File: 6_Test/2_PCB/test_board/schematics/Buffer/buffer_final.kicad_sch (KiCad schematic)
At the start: 12 parts, among them J11 Buffer_PWR_Jumper, U7 SN74ALVCH162827DLR

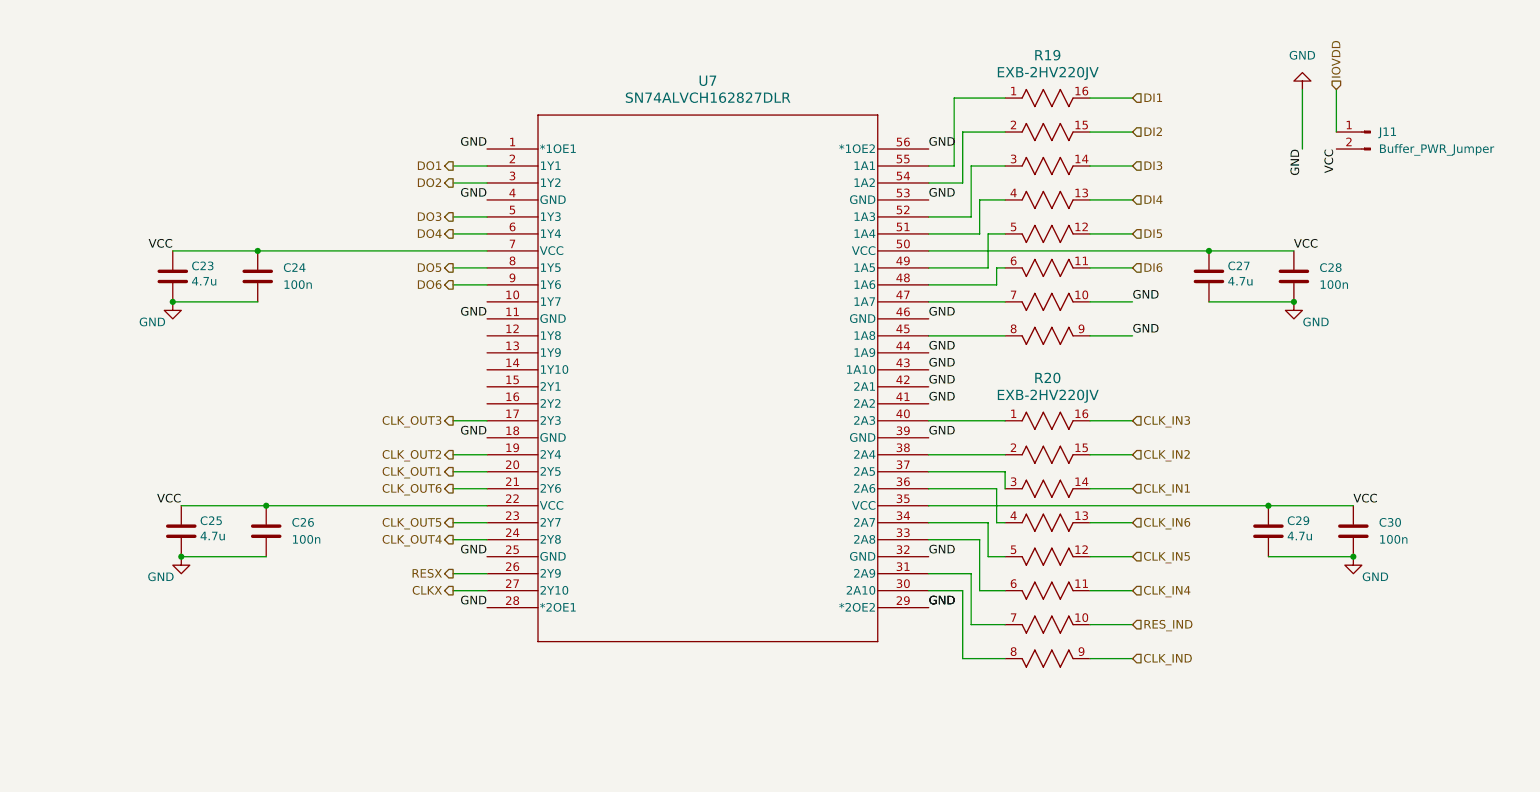
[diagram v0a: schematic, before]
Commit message: Finished board layout
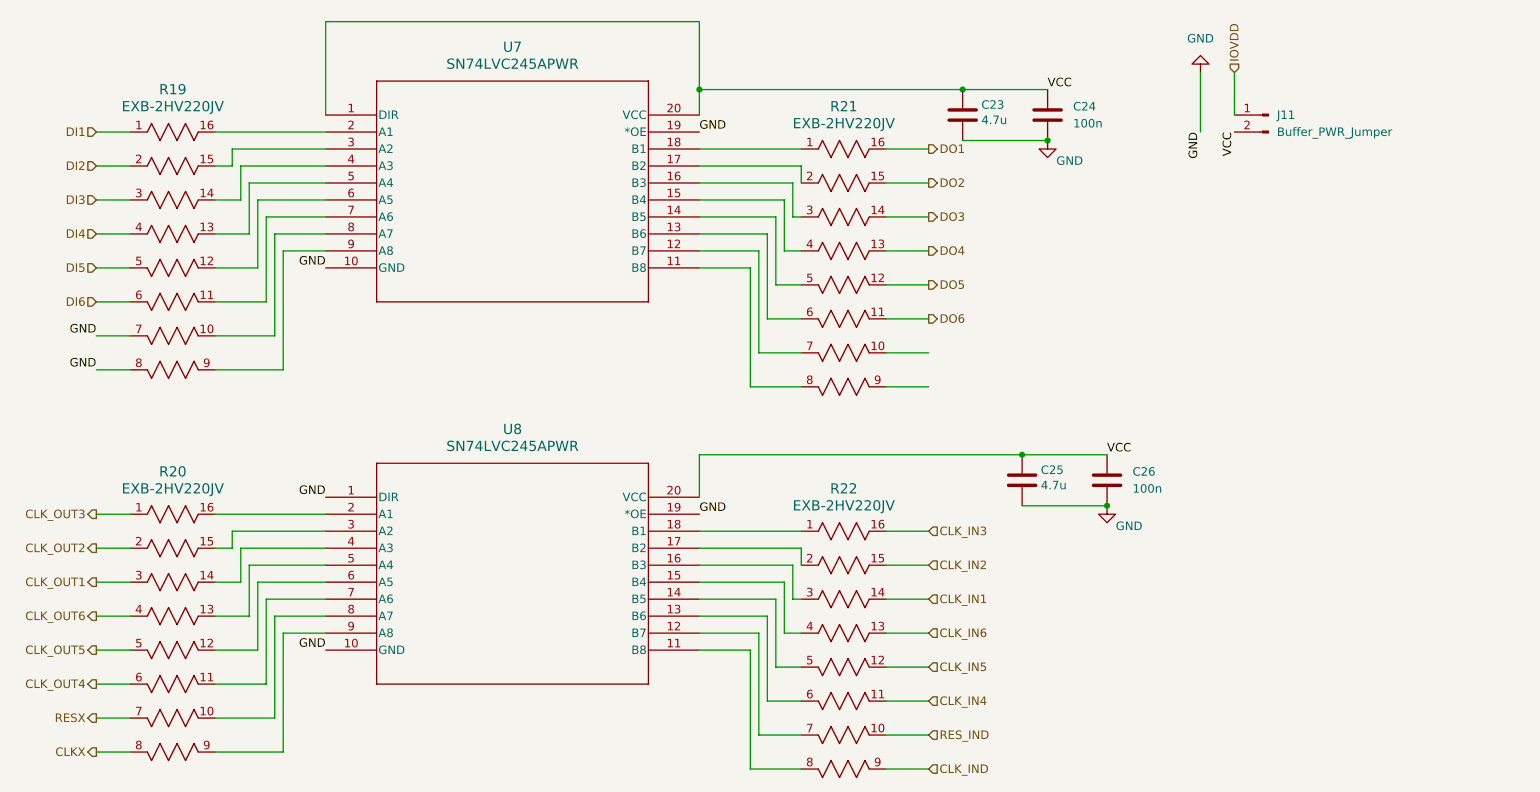
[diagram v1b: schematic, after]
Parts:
- removed C27, C29: 4.7u, Capacitor_SMD:C_0603_1608Metric, symbol Device:C
- removed C28, C30: 100n, Capacitor_SMD:C_0402_1005Metric, symbol Device:C
- removed U7: SN74ALVCH162827DLR, 74ALVCHFootprints:DL56, symbol 74ALVCH:SN74ALVCH162827DLR
- added R21, R22: EXB-2HV220JV, 22res_arrayFootprints:RES_EXB2HV, symbol 22res_array:EXB-2HV220JV
- added U7: SN74LVC245APWR, SN74LVC245APWRFootprints:PW20, symbol SN74LVC245APWR:SN74LVC245APWR
- added U8: SN74LVC245APWR, PW20, symbol SN74LVC245APWR:SN74LVC245APWR
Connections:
- net CLKX: now also R20.8
- net CLK_IN1: now also R22.14; no longer R20.14
- net CLK_IN2: now also R22.15; no longer R20.15
- net CLK_IN3: now also R22.16; no longer R20.16
- net CLK_IN4: now also R22.11; no longer R20.11
- net CLK_IN5: now also R22.12; no longer R20.12
- net CLK_IN6: now also R22.13; no longer R20.13
- net CLK_IND: now also R22.9; no longer R20.9
- net CLK_OUT1: now also R20.3
- net CLK_OUT2: now also R20.2
- net CLK_OUT3: now also R20.1
- net CLK_OUT4: now also R20.6
- net CLK_OUT5: now also R20.5
- net CLK_OUT6: now also R20.4
- net DI1: now also R19.1; no longer R19.16
- net DI2: now also R19.2; no longer R19.15
- net DI3: now also R19.3; no longer R19.14
- net DI4: now also R19.4; no longer R19.13
- net DI5: now also R19.5; no longer R19.12
- net DI6: now also R19.6; no longer R19.11
- net DO1: now also R21.16
- net DO2: now also R21.15
- net DO3: now also R21.14
- net DO4: now also R21.13
- net DO5: now also R21.12
- net DO6: now also R21.11
- net GND: now also R19.7, R19.8, U7.10 (GND), U7.19 (*OE), U8.1 (DIR), U8.10 (GND), U8.19 (*OE); no longer R19.10, R19.9
- net RESX: now also R20.7
- net RES_IND: now also R22.10; no longer R20.10
- net VCC: now also U7.1 (DIR), U7.20 (VCC), U8.20 (VCC)
- new net: R19.10, U7.8 (A7)
- new net: R19.11, U7.7 (A6)
- new net: R19.12, U7.6 (A5)
- new net: R19.13, U7.5 (A4)
- new net: R19.14, U7.4 (A3)
- new net: R19.15, U7.3 (A2)
- new net: R19.16, U7.2 (A1)
- new net: R19.9, U7.9 (A8)
- new net: R20.10, U8.8 (A7)
- new net: R20.11, U8.7 (A6)
- new net: R20.12, U8.6 (A5)
- new net: R20.13, U8.5 (A4)
- new net: R20.14, U8.4 (A3)
- new net: R20.15, U8.3 (A2)
- new net: R20.16, U8.2 (A1)
- new net: R20.9, U8.9 (A8)
- new net: R21.1, U7.18 (B1)
- new net: R21.2, U7.17 (B2)
- new net: R21.3, U7.16 (B3)
- new net: R21.4, U7.15 (B4)
- new net: R21.5, U7.14 (B5)
- new net: R21.6, U7.13 (B6)
- new net: R21.7, U7.12 (B7)
- new net: R21.8, U7.11 (B8)
- new net: R22.1, U8.18 (B1)
- new net: R22.2, U8.17 (B2)
- new net: R22.3, U8.16 (B3)
- new net: R22.4, U8.15 (B4)
- new net: R22.5, U8.14 (B5)
- new net: R22.6, U8.13 (B6)
- new net: R22.7, U8.12 (B7)
- new net: R22.8, U8.11 (B8)
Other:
- moved on the sheet: J11
